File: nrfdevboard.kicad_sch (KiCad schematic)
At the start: 15 parts, among them J1 USB2.0, J3 Conn_01x17_Pin, J4 Conn_01x17_Pin, U1 MDBT50Q-P1MV2, Y1 32.768

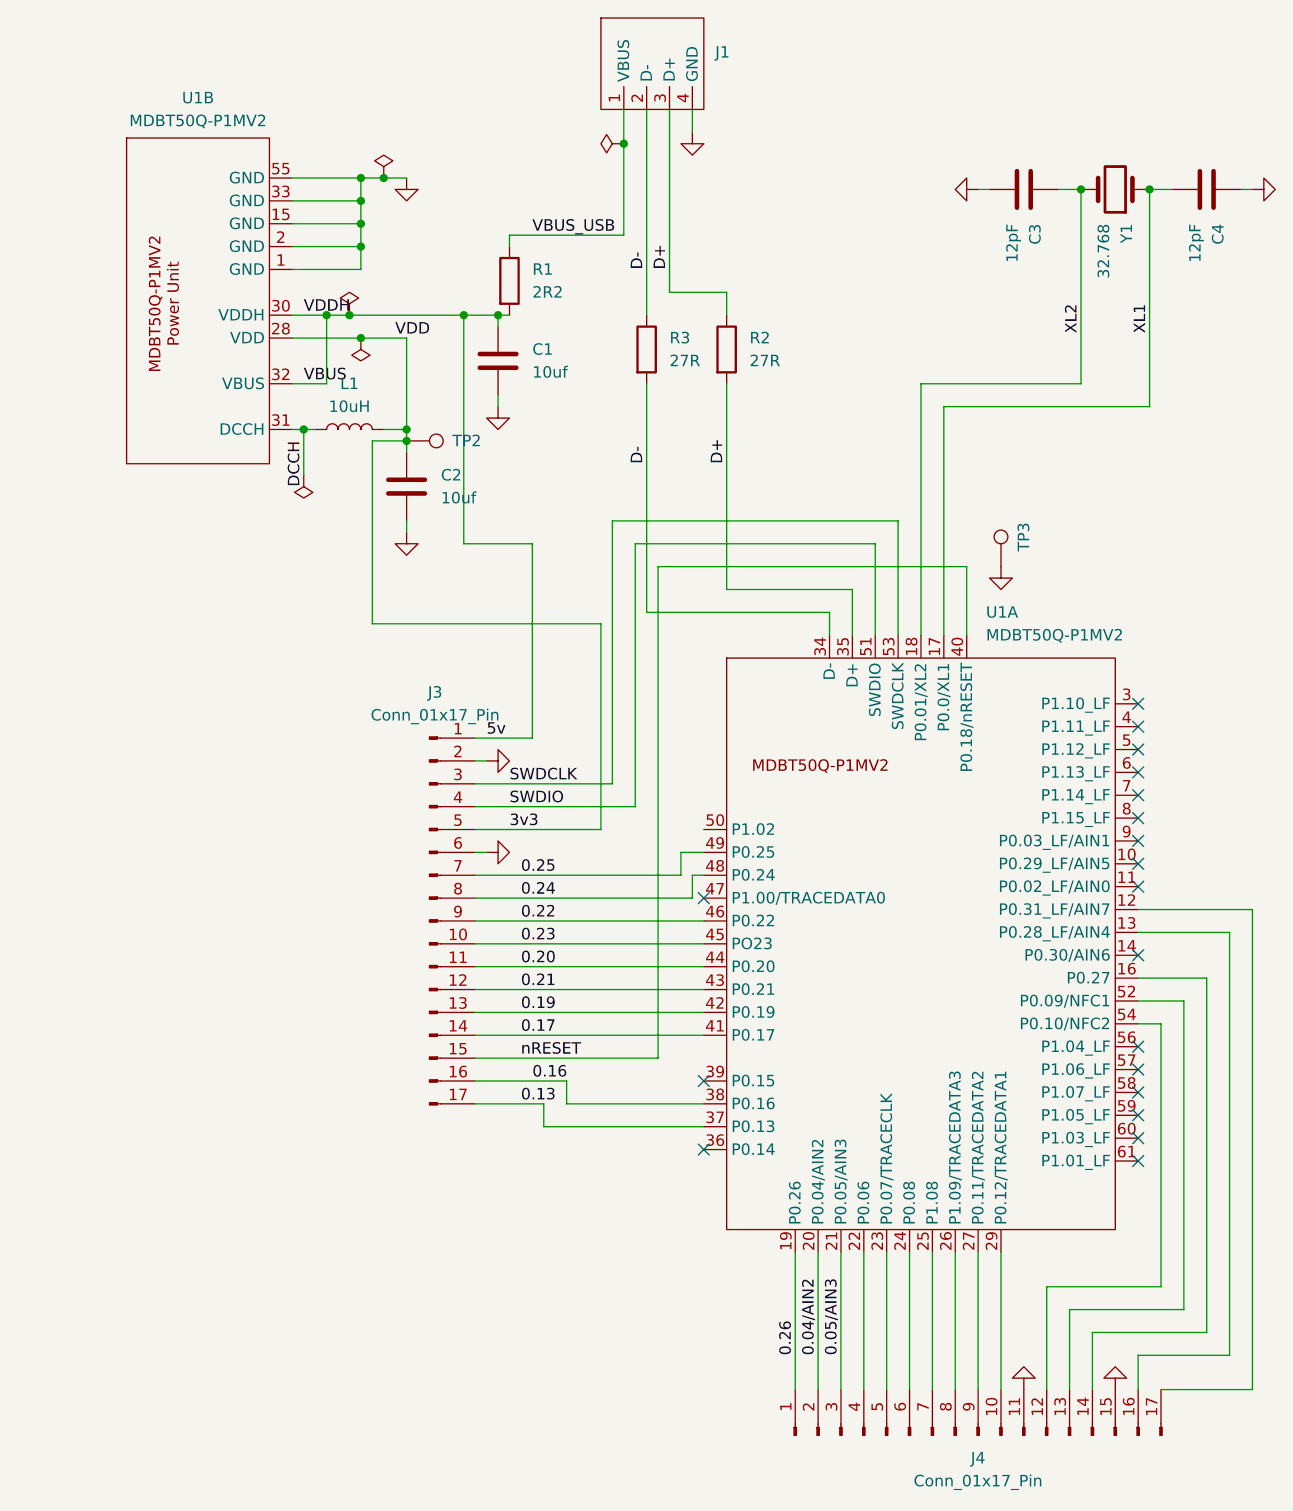
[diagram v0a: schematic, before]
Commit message: Finished p1
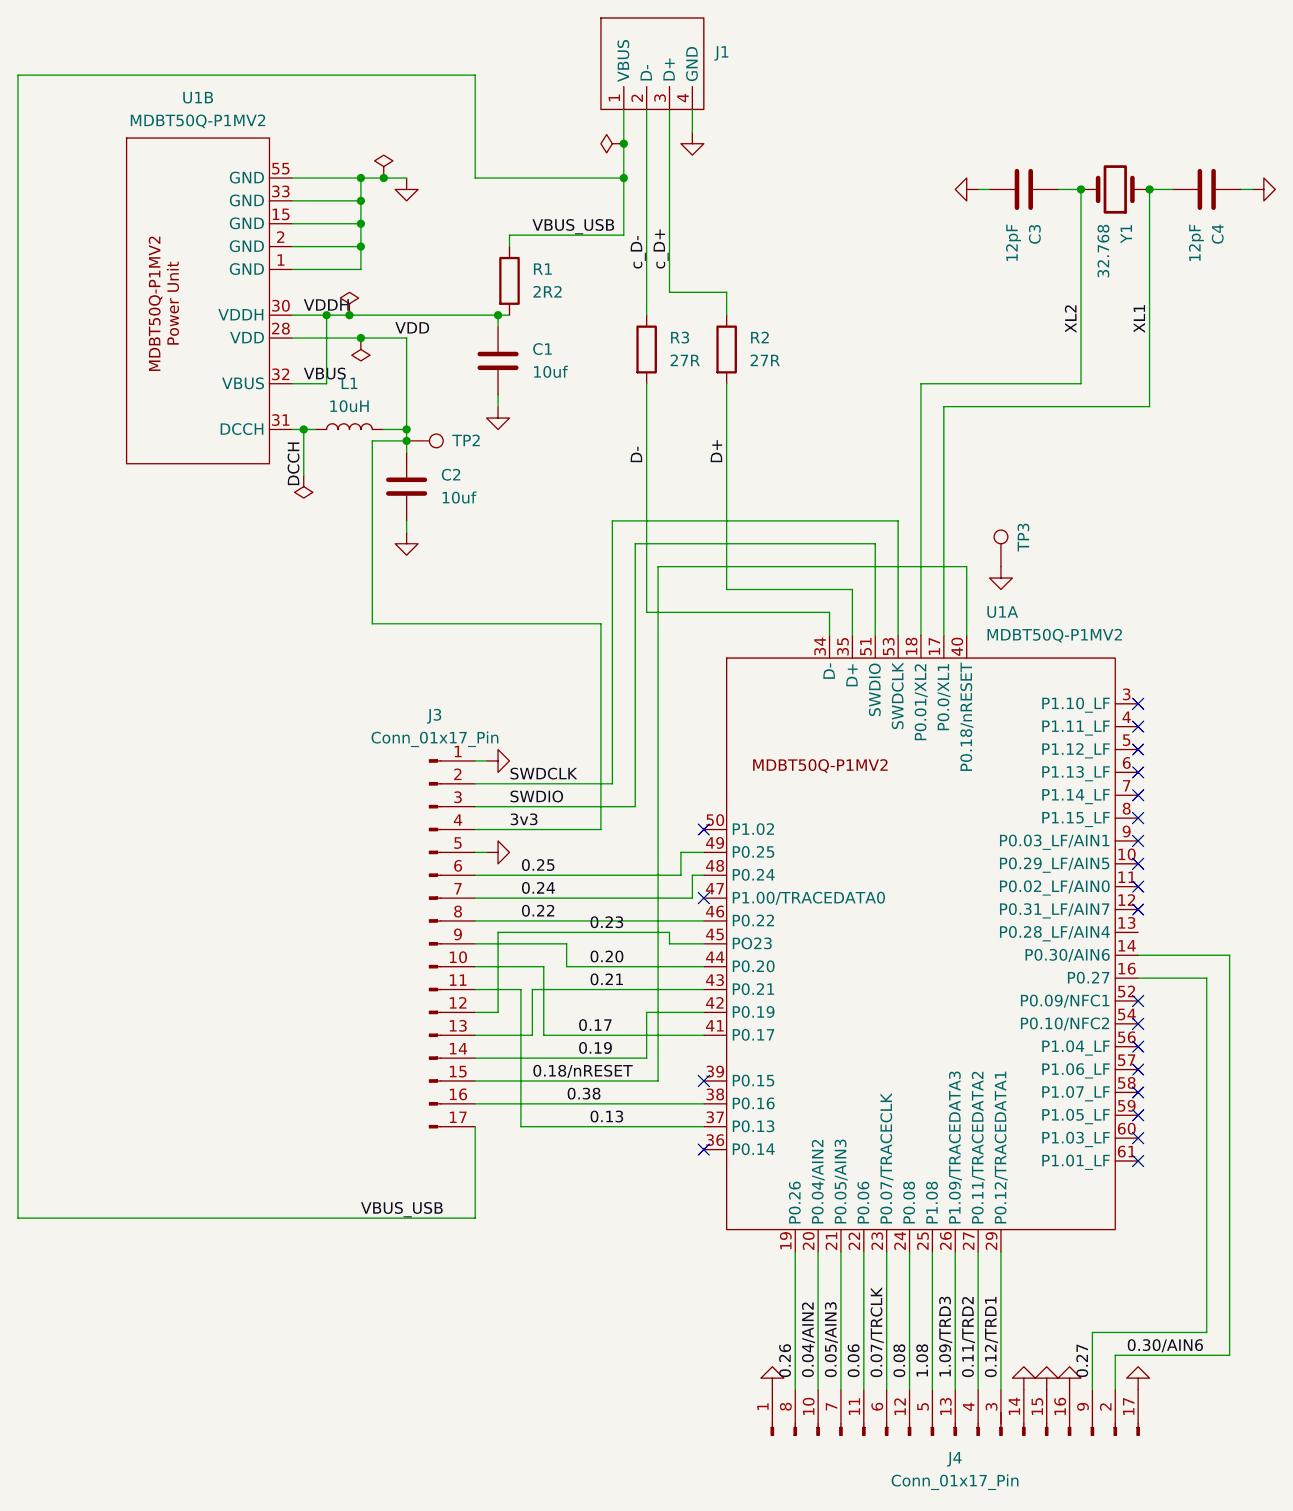
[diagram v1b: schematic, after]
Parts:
- J1: footprint TH-A1OC:th_pogo_pins_4 -> Connector_USB:USB_A_Kycon_KUSBX-AS1N-B_Horizontal
- J3: footprint (none) -> Connector_Samtec_HPM_THT:Samtec_HPM-17-01-x-S_Straight_1x17_Pitch5.08mm
- J4: footprint (none) -> Connector_Samtec_HPM_THT:Samtec_HPM-17-01-x-S_Straight_1x17_Pitch5.08mm; symbol Connector:Conn_01x17_Pin -> nrfdevboard:Conn_01x17_Pin
- U1: footprint TH-A1OC:TH_MDBT50Q-P1MV2 -> TH1:TH_MDBT50Q-P1MV2
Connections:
- net 0.04/AIN2: now also J4.10 (Pin_10); no longer J4.2 (Pin_2)
- net 0.05/AIN3: now also J4.7 (Pin_7); no longer J4.3 (Pin_3)
- net 0.13: now also J3.11 (Pin_11); no longer J3.17 (Pin_17)
- net 0.17: now also J3.10 (Pin_10); no longer J3.14 (Pin_14)
- net 0.19: now also J3.14 (Pin_14); no longer J3.13 (Pin_13)
- net 0.20: now also J3.9 (Pin_9); no longer J3.11 (Pin_11)
- net 0.21: now also J3.13 (Pin_13); no longer J3.12 (Pin_12)
- net 0.22: now also J3.8 (Pin_8); no longer J3.9 (Pin_9)
- net 0.23: now also J3.12 (Pin_12); no longer J3.10 (Pin_10)
- net 0.24: now also J3.7 (Pin_7); no longer J3.8 (Pin_8)
- net 0.25: now also J3.6 (Pin_6); no longer J3.7 (Pin_7)
- net 0.26: now also J4.8 (Pin_8); no longer J4.1 (Pin_1)
- net 3v3: now also J3.4 (Pin_4); no longer J3.5 (Pin_5)
- net D+: no longer J1.3 (D+), R2.1
- net D-: no longer J1.2 (D-), R3.1
- net GND: now also J3.1 (Pin_1), J3.5 (Pin_5), J4.1 (Pin_1), J4.14 (Pin_14), J4.16 (Pin_16), J4.17 (Pin_17); no longer J3.2 (Pin_2), J3.6 (Pin_6), J4.11 (Pin_11)
- net SWDCLK: now also J3.2 (Pin_2); no longer J3.3 (Pin_3)
- net SWDIO: now also J3.3 (Pin_3); no longer J3.4 (Pin_4)
- net VBUS_USB: now also J3.17 (Pin_17)
- net at U1.12 (P0.31_LF/AIN7): no longer J4.17 (Pin_17)
- net at U1.13 (P0.28_LF/AIN4): no longer J4.16 (Pin_16)
- net 0.30/AIN6: now reaches U1.14 (P0.30/AIN6)
- net 0.30/AIN6: now also J4.2 (Pin_2)
- net 0.27: now reaches U1.16 (P0.27)
- net 0.27: now also J4.9 (Pin_9); no longer J4.14 (Pin_14)
- net 0.06: now reaches U1.22 (P0.06)
- net 0.06: now also J4.11 (Pin_11); no longer J4.4 (Pin_4)
- net 0.07/TRCLK: now reaches U1.23 (P0.07/TRACECLK)
- net 0.07/TRCLK: now also J4.6 (Pin_6); no longer J4.5 (Pin_5)
- net 0.08: now reaches U1.24 (P0.08)
- net 0.08: now also J4.12 (Pin_12); no longer J4.6 (Pin_6)
- net 1.08: now reaches U1.25 (P1.08)
- net 1.08: now also J4.5 (Pin_5); no longer J4.7 (Pin_7)
- net 1.09/TRD3: now reaches U1.26 (P1.09/TRACEDATA3)
- net 1.09/TRD3: now also J4.13 (Pin_13); no longer J4.8 (Pin_8)
- net 0.11/TRD2: now reaches U1.27 (P0.11/TRACEDATA2)
- net 0.11/TRD2: now also J4.4 (Pin_4); no longer J4.9 (Pin_9)
- net 0.12/TRD1: now reaches U1.29 (P0.12/TRACEDATA1)
- net 0.12/TRD1: now also J4.3 (Pin_3); no longer J4.10 (Pin_10)
- net at U1.52 (P0.09/NFC1): no longer J4.13 (Pin_13)
- net at U1.54 (P0.10/NFC2): no longer J4.12 (Pin_12)
- net 0.16 renamed 0.38
- net 5v renamed VBUS
- net VBUS: no longer J3.1 (Pin_1)
- net nRESET renamed 0.18/nRESET
- new net c_D+: J1.3 (D+), R2.1
- new net c_D-: J1.2 (D-), R3.1
- no-connect marks 19 -> 22
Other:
- moved on the sheet: J3, J4
